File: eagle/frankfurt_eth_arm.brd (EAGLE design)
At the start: 71.6 x 65.1 mm, 78 parts, among them IC1 STM32F103C6T7A, IC2 ENC28J60-SO, IC3 SN65HVD232, IC4 LM2575S, IC5 11AA02E48, IC6 MCP23A256, IC7 AT45DB041D, J2 A00-108-220-450, J5 TAMPER, X1 8 MHz, X2 32768 hZ, X3 25 MHz

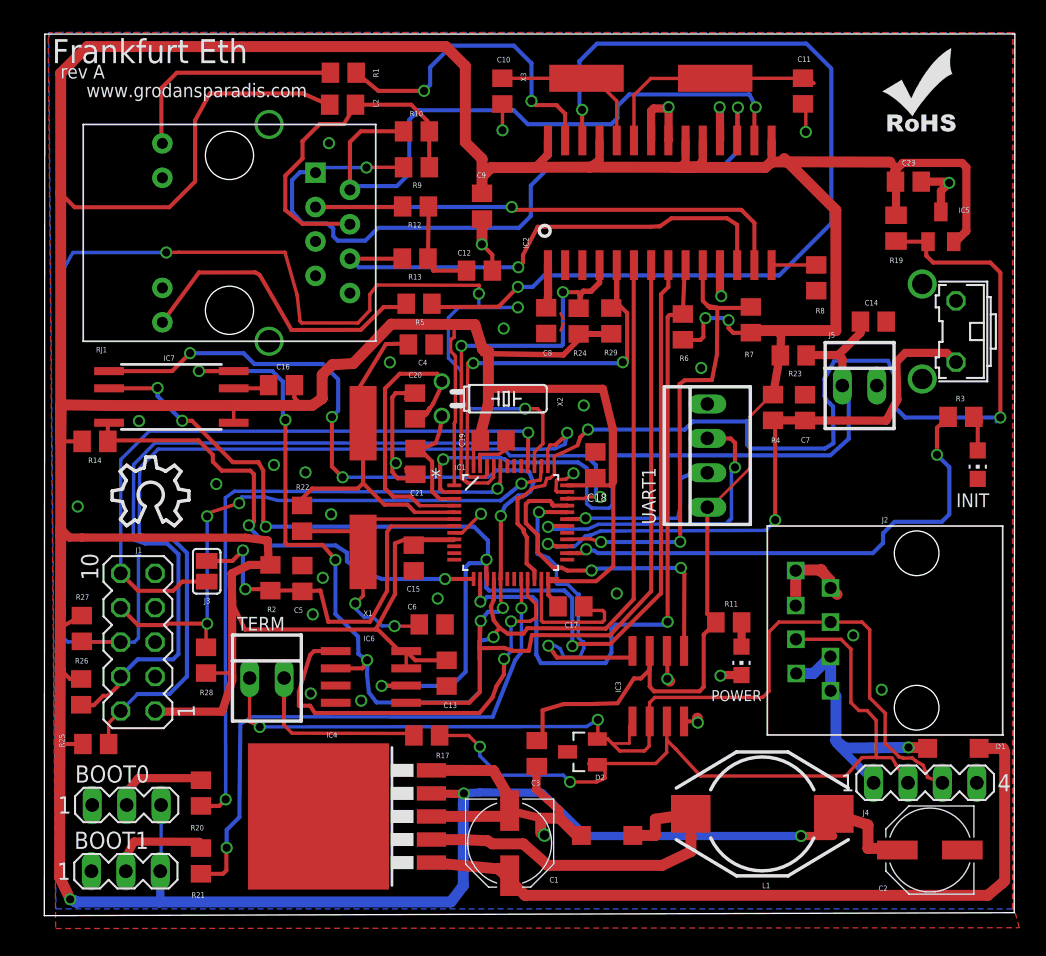
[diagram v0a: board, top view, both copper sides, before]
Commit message: Added Gerbers
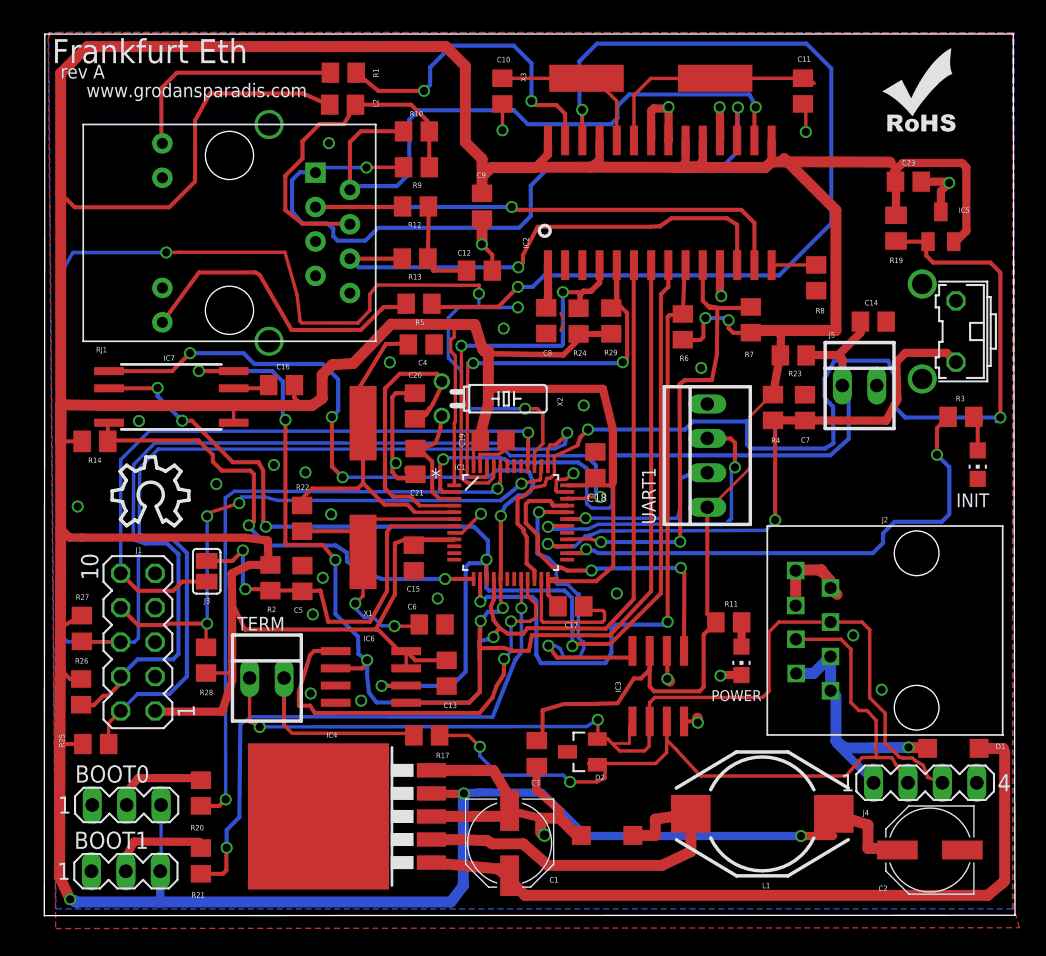
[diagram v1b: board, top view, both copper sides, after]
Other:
- board size 71.6 x 65.1 mm -> 71.7 x 65.1 mm
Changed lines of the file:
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@@
 <text x="69.74" y="31.16" size="1.016" layer="25" rot="R180">INIT</text>
 <wire x1="-0.01" y1="-0.01" x2="0.03" y2="65.06" width="0" layer="20"/>
-<wire x1="0.03" y1="65.06" x2="71.63" y2="65.07" width="0" layer="20"/>
-<wire x1="71.63" y1="65.07" x2="71.58" y2="0.21" width="0" layer="20"/>
-<wire x1="71.58" y1="0.21" x2="-0.01" y2="-0.01" width="0" layer="20"/>
+<wire x1="0.03" y1="65.06" x2="71.51" y2="65.07" width="0" layer="20"/>
+<wire x1="71.51" y1="65.07" x2="71.64" y2="0.02" width="0" layer="20"/>
+<wire x1="71.64" y1="0.02" x2="-0.01" y2="-0.01" width="0" layer="20"/>
 <circle x="36.93" y="50.54" radius="0.1220625" width="0.8128" layer="25"/>
 </plain>
